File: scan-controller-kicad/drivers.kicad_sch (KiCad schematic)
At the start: 18 parts, among them CN4 Lamp, CN5 Fan, CN6 Motor, Q1 IRF7470, Q5 BC817, U5 DRV8871DDA

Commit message: Adding missing components Mfnrs and footprints
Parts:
- C7: LCSC C267472 -> C267472
- CN4, CN5: LCSC (none) -> C475125; LCSC Part C475125 -> (none)
- CN6: LCSC (none) -> C475144; LCSC Part C475144 -> (none)

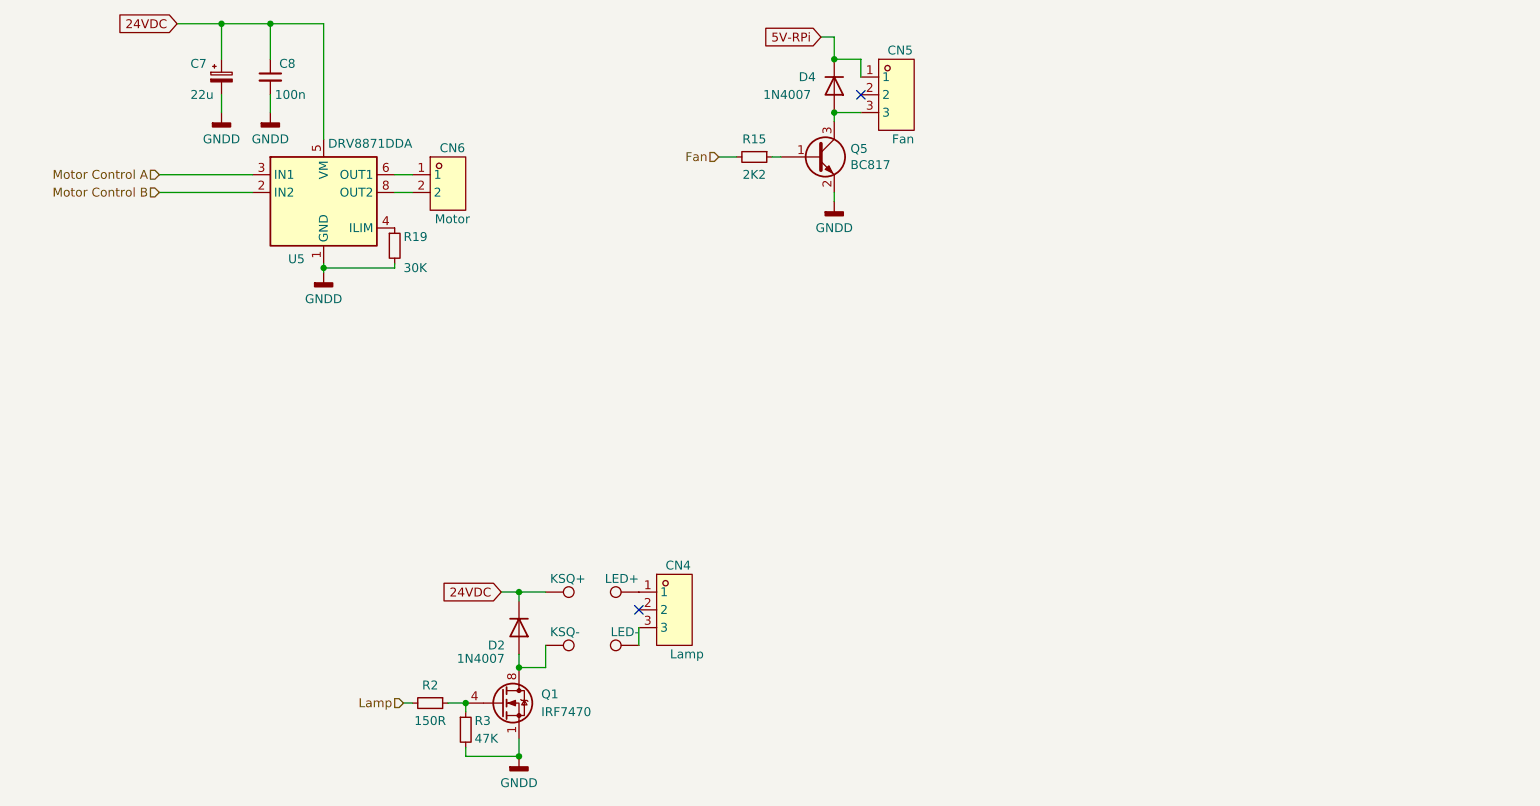
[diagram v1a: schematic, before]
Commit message: Adding Constant Current LED Driver
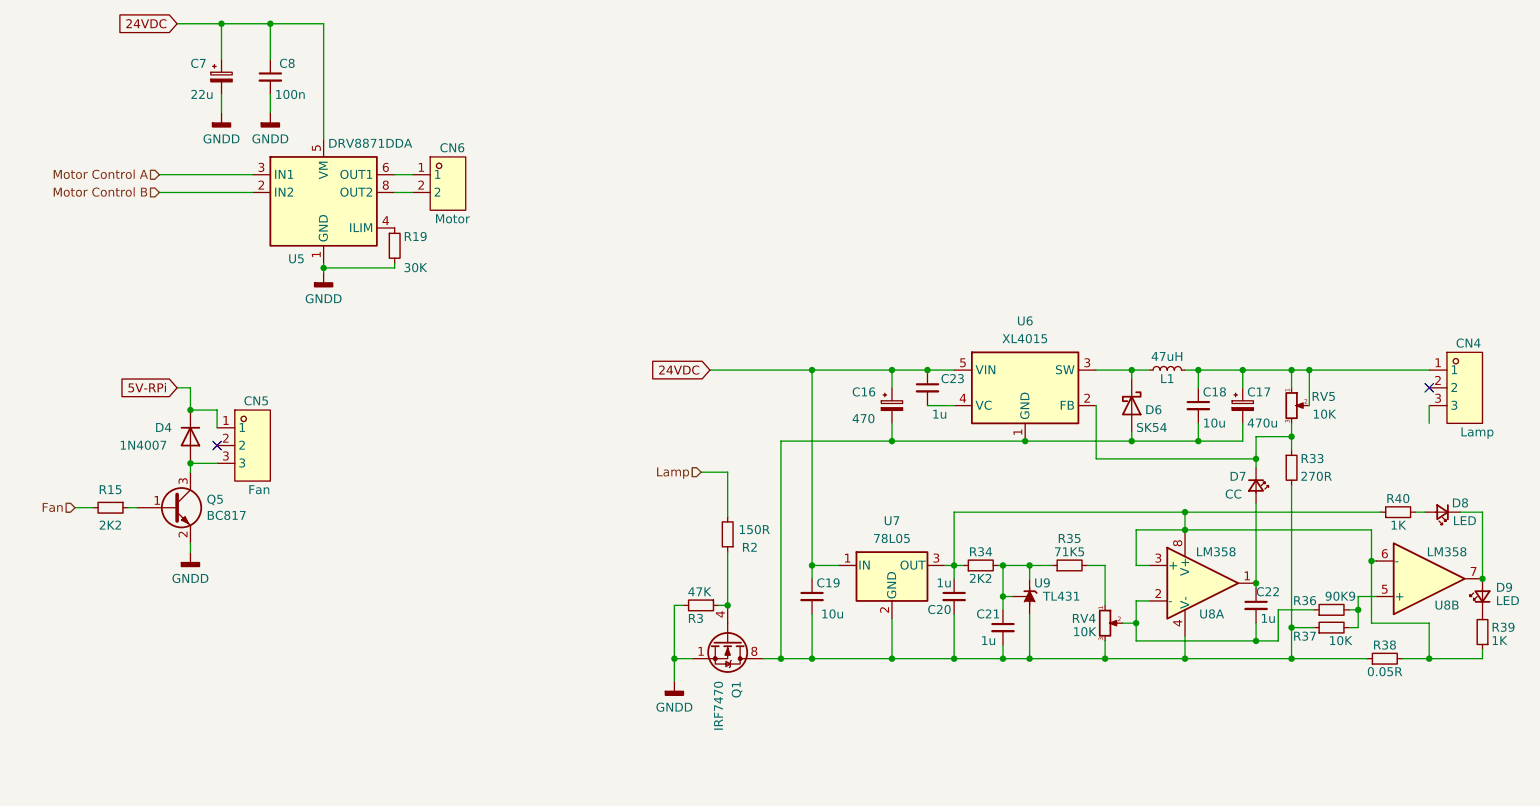
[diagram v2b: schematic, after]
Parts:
- removed D2: 1N4007, Diode_SMD:D_SOD-123F, symbol Diode:1N4001
- removed TP1: KSQ+, TestPoint:TestPoint_THTPad_D3.0mm_Drill1.5mm, symbol Connector:TestPoint
- removed TP2: KSQ-, TestPoint:TestPoint_THTPad_D3.0mm_Drill1.5mm, symbol Connector:TestPoint
- removed TP4: LED+, TestPoint:TestPoint_THTPad_D3.0mm_Drill1.5mm, symbol Connector:TestPoint
- removed TP5: LED-, TestPoint:TestPoint_THTPad_D3.0mm_Drill1.5mm, symbol Connector:TestPoint
- added C16: 470, symbol Device:C_Polarized_Small
- added C17: 470u, symbol Device:C_Polarized_Small
- added C18, C19: 10u, symbol Device:C_Small
- added C20, C21, C22, C23: 1u, symbol Device:C_Small
- added D6: SK54, symbol Device:D_Schottky
- added D7: CC, symbol Device:LED_Small
- added D8, D9: LED, symbol Device:LED_Small
- added L1: 47uH, symbol Device:L_Small
- added R33: 270R, symbol Device:R_Small
- added R34: 2K2, symbol Device:R_Small
- added R35: 71K5, symbol Device:R_Small
- added R36: 90K9, symbol Device:R_Small
- added R37: 10K, symbol Device:R_Small
- added R38: 0.05R, symbol Device:R_Small
- added R39, R40: 1K, symbol Device:R_Small
- added RV4, RV5: 10K, symbol Device:R_Potentiometer_Small
- added U6: XL4015, Package_TO_SOT_SMD:TO-263-5_TabPin3, symbol Regulator_Switching:XL4015
- added U7: 78L05, symbol Regulator_Linear:L7805
- added U8: LM358, symbol Amplifier_Operational:LM358
- added U9: TL431, Package_TO_SOT_SMD:SOT-23, symbol Reference_Voltage:TL431DBZ
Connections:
- net 24VDC: now also C16.1, C19.1, C23.1, U6.5 (VIN), U7.1 (IN)
- net at CN4.1: now also C17.1, C18.1, L1.2, RV5.1, RV5.2
- net at Q1.5 (D), Q1.6 (D), Q1.7 (D)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: now also C16.2, C17.2, C18.2, C19.2, C20.2, C21.2, D6.2 (A), R33.2, R37.1, R38.1, RV4.3, U6.1 (GND), U7.2 (GND), U8.4 (V-), U9.3 (A)
- new net: D6.1 (K), L1.1, U6.3 (SW)
- new net: D8.1 (K), D9.2 (A), U8.7
- new net: D8.2 (A), R40.2
- new net: C20.1, R34.1, R38.2, R39.1, R40.1, U7.3 (OUT), U8.3 (+), U8.6 (-), U8.8 (V+)
- new net: C21.1, R34.2, R35.1, U9.1 (K), U9.2 (REF)
- new net: R36.2, R37.2, U8.5 (+)
- new net: D7.1 (K), R33.1, RV5.3, U6.2 (FB)
- new net: R35.2, RV4.1
- new net: C22.2, R36.1, RV4.2, U8.2 (-)
- new net: C22.1, D7.2 (A), U8.1
- new net: D9.1 (K), R39.2
- new net: C23.2, U6.4 (VC)
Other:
- moved on the sheet: CN4, CN5, D4, Q1, Q5, R15, R2, R3
